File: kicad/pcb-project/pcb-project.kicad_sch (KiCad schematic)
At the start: 13 parts, among them J1 LOGIC CONN, U1 74HC237

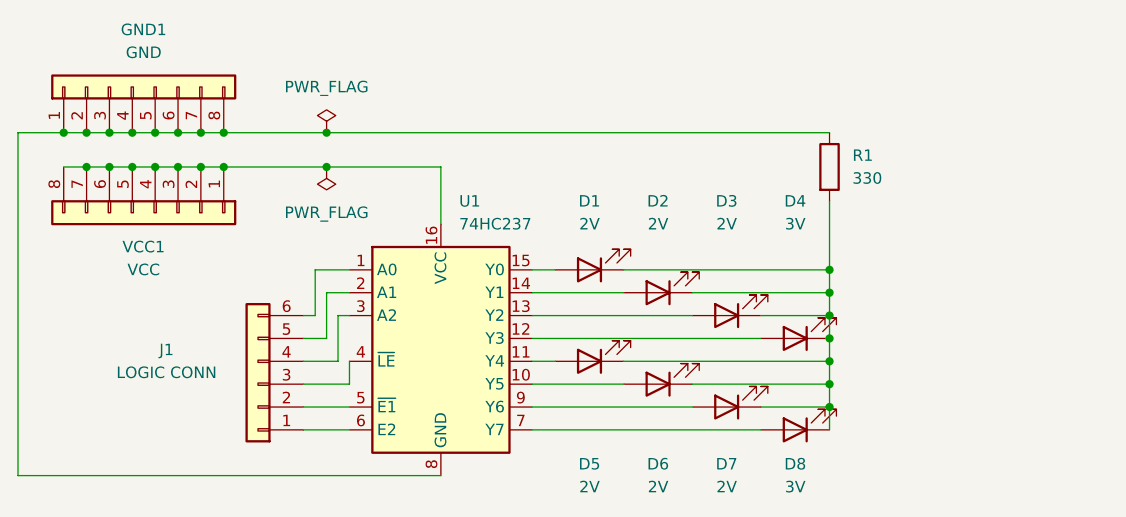
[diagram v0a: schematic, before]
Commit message: finish pcb
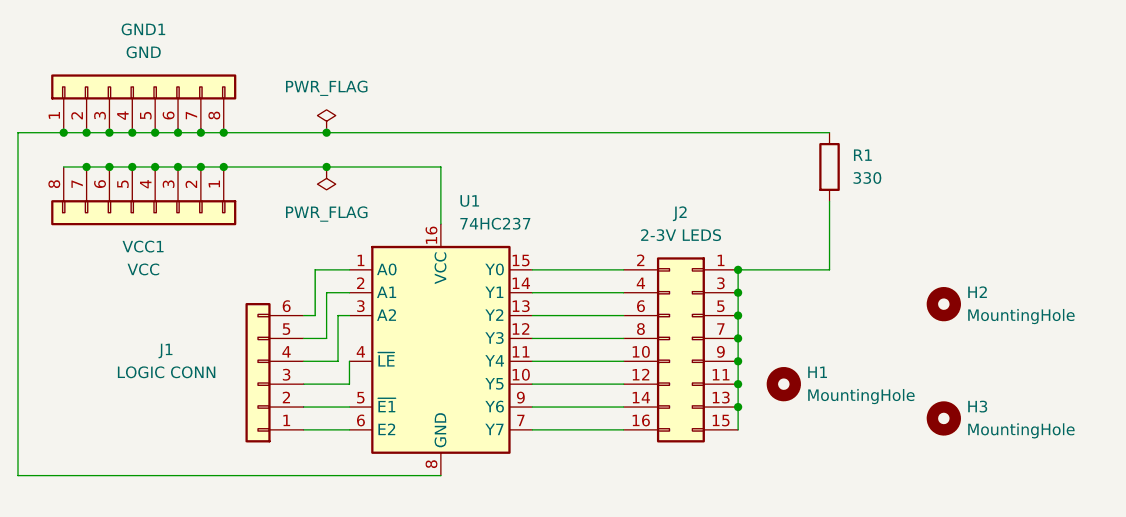
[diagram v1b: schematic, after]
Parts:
- removed D1, D2, D3, D5, D6, D7: 2V, Connector_PinSocket_2.54mm:PinSocket_1x02_P2.54mm_Vertical, symbol Device:LED
- removed D4, D8: 3V, Connector_PinSocket_2.54mm:PinSocket_1x02_P2.54mm_Vertical, symbol Device:LED
- added H1, H2, H3: MountingHole, MountingHole:MountingHole_3.2mm_M3, symbol Mechanical:MountingHole
- added J2: 2-3V LEDS, Connector_PinSocket_2.54mm:PinSocket_2x08_P2.54mm_Vertical, symbol Connector_Generic:Conn_02x08_Odd_Even
- R1: footprint Resistor_THT:R_Axial_DIN0204_L3.6mm_D1.6mm_P1.90mm_Vertical -> Resistor_THT:R_Axial_Power_L25.0mm_W9.0mm_P10.16mm_Vertical
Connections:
- net at R1.2: now also J2.1 (Pin_1), J2.11 (Pin_11), J2.13 (Pin_13), J2.15 (Pin_15), J2.3 (Pin_3), J2.5 (Pin_5), J2.7 (Pin_7), J2.9 (Pin_9)
- net at U1.7 (Y7): now also J2.16 (Pin_16)
- net at U1.11 (Y4): now also J2.10 (Pin_10)
- net at U1.10 (Y5): now also J2.12 (Pin_12)
- net at U1.12 (Y3): now also J2.8 (Pin_8)
- net at U1.13 (Y2): now also J2.6 (Pin_6)
- net at U1.14 (Y1): now also J2.4 (Pin_4)
- net at U1.15 (Y0): now also J2.2 (Pin_2)
- net at U1.9 (Y6): now also J2.14 (Pin_14)
